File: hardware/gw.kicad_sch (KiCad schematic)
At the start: 21 parts, among them J1 USB_OTG, J2 Conn_01x04, U1 ESP-12F, U2 Ai-Thinker-Ra-02, U3 AMS1117-3.3

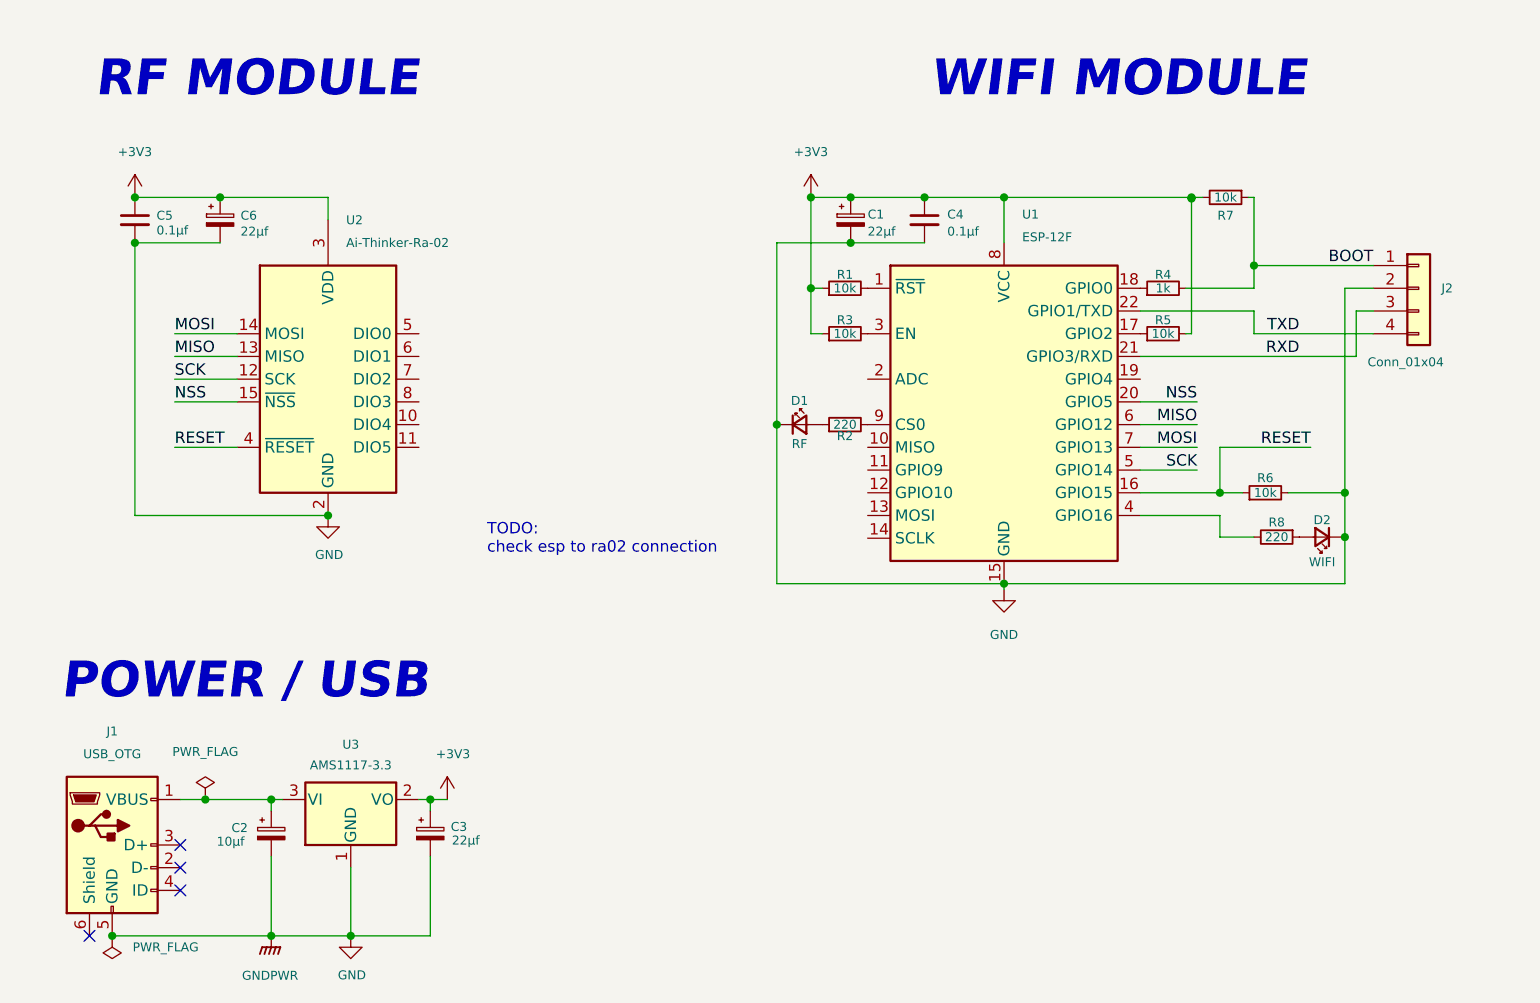
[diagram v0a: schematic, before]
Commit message: Update schematics, almost fab ready
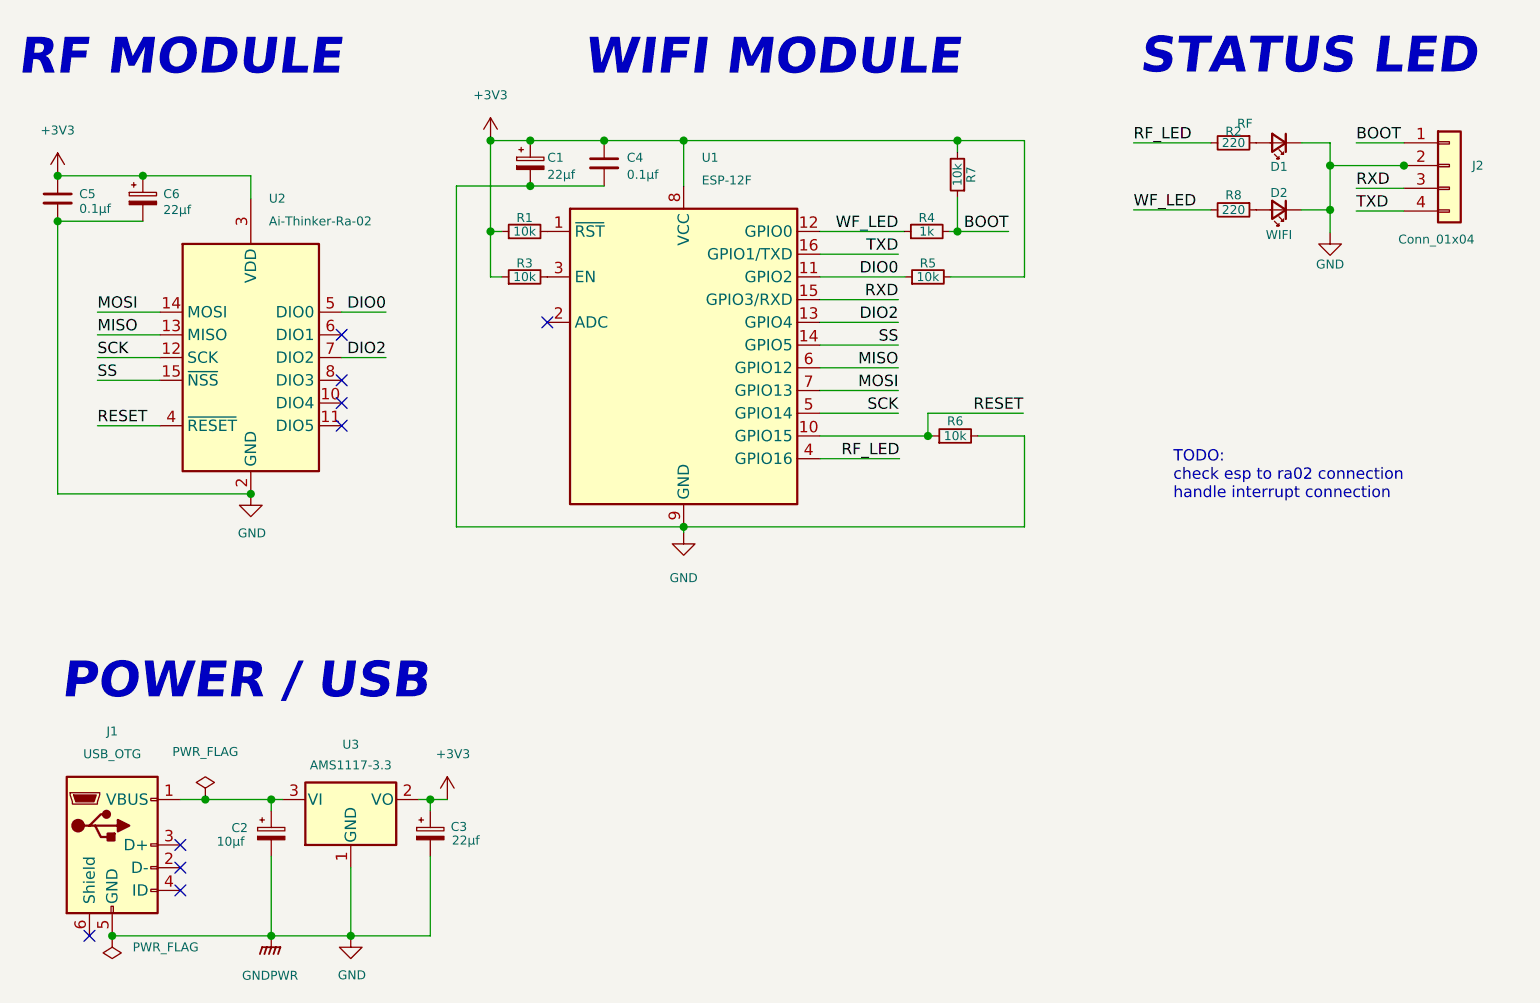
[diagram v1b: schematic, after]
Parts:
- U1: footprint RF_Module:ESP-12E -> RF_Module:ESP-07; symbol RF_Module:ESP-12F -> RF_Module:ESP-07
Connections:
- net GND: now also U1.9 (GND); no longer U1.15 (GND)
- net RESET: now also U1.10 (GPIO15); no longer U1.16 (GPIO15)
- net RXD: now also U1.15 (GPIO3/RXD); no longer U1.21 (GPIO3/RXD)
- net TXD: now also U1.16 (GPIO1/TXD); no longer U1.22 (GPIO1/TXD)
- net RF_LED: now reaches R2.2
- net RF_LED: now also U1.4 (GPIO16); no longer U1.9 (CS0)
- net WF_LED: now reaches R8.2
- net WF_LED: now also R4.1, U1.12 (GPIO0); no longer U1.4 (GPIO16)
- net DIO0: now reaches U2.5 (DIO0)
- net DIO0: now also R5.1, U1.11 (GPIO2)
- net DIO2: now reaches U2.7 (DIO2)
- net DIO2: now also U1.13 (GPIO4)
- net SS: now reaches U1.14 (GPIO5)
- net SS: now also U2.15 (~{NSS})
- removed net NSS: U1.20 (GPIO5), U2.15 (~{NSS})
- no-connect marks 4 -> 9
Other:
- note added: "STATUS LED"
- note added: "TODO: check esp to ra02 connection handle interrupt connection"
- note removed: "TODO: check esp to ra02 connection"
- moved on the sheet: C1, C4, C5, C6, D1, D2, J2, R1, R2, R3, R4, R5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
